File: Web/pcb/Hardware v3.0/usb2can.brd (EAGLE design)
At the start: 59 x 15.8 mm, 49 parts, among them CON1 USB_A_MALESMD, IC1 ADM3053M, IC2 LD1117S33

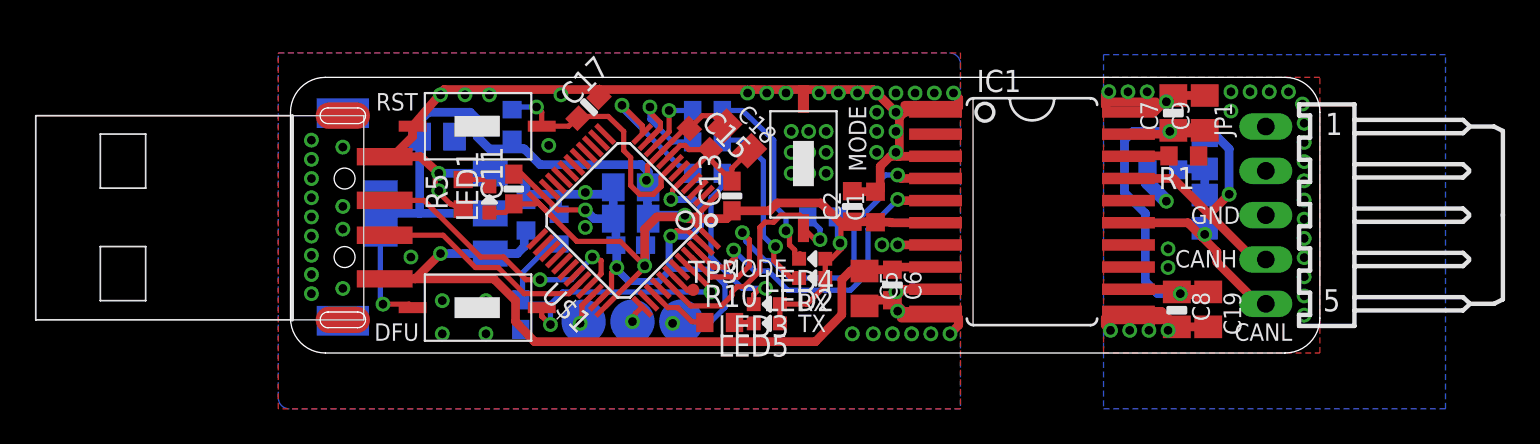
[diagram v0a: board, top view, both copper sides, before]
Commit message: updates
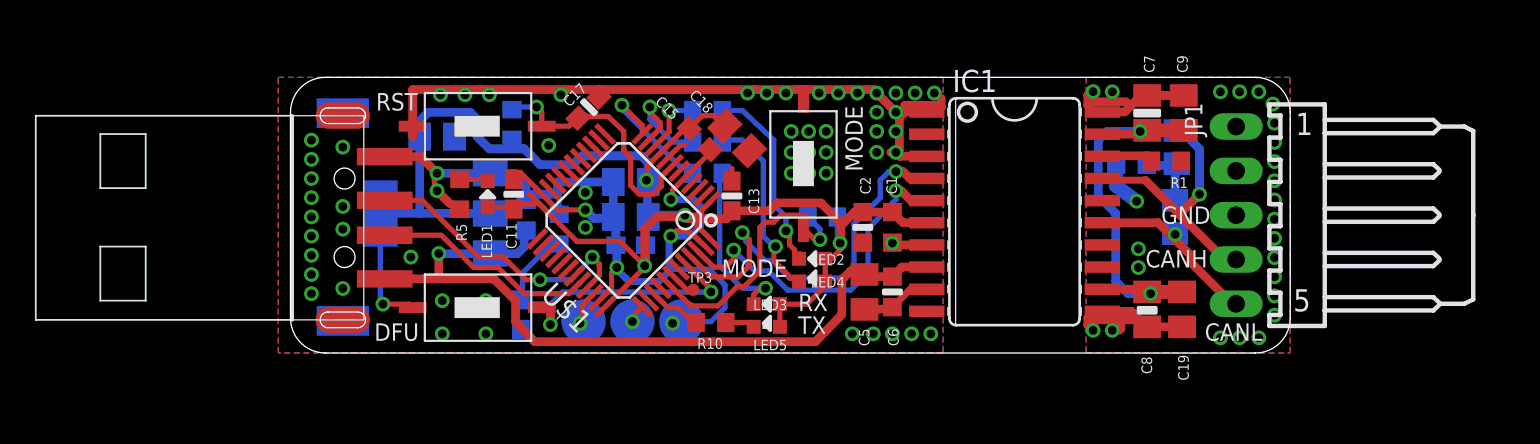
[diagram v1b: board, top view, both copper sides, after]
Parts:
- IC1: value ADM3053M -> ADM3053; device ADM3053:SO20W -> ADM3053:SO20L
- moved C10 1.82 mm to (48.2, 10.8)
- moved R2 1.73 mm to (50.7, 7.80)
- moved C8 1.70 mm to (49.1, 2.50)
- moved JP1 1.70 mm to (54.2, 7.90)
- moved R3 1.63 mm to (50.8, 11.8)
- moved C1 1.52 mm to (34.5, 7.20), turned to 270 degrees
- moved C19 1.50 mm to (51.1, 2.50)
- moved C7 1.50 mm to (49.1, 13.8)
- moved C2 1.34 mm to (32.8, 7.20), turned to 270 degrees
- moved C9 1.20 mm to (51.2, 13.8)
- moved R1 1.04 mm to (50.2, 11.0)
- moved IC1 1.00 mm to (41.5, 8.10)
- moved U$2 0.90 mm to (41.5, 11.9)
- moved R10 0.50 mm to (24.1, 1.75)
- moved C6 0.40 mm to (34.5, 3.50)
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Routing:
- net GND: track 126.9 -> 108.0 mm, vias 68 -> 63
- net N$1: track 2.33 -> 3.47 mm
- net CANH: track 15.9 -> 16.7 mm
- net N$4: track 3.05 -> 3.77 mm
- net N$17: track 1.12 -> 1.80 mm
- net VCC: track 44.9 -> 44.2 mm
- net GNDA: track 20.6 -> 20.0 mm, vias 28 -> 25
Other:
- board size 59 x 15.8 mm -> 57.3 x 15.8 mm
- board text added: "2019"
- board text added: "HW:Daniel Sascha"
- board text added: "Rev. 4"
- board text added: "modm.io"
- board text removed: "2017"
- board text removed: "HW: Daniel"
- board text removed: "Rev. 3"
- board text removed: "xpcc.io"
